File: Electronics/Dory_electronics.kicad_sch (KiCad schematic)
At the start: 12 parts, among them J1 Bateria 2s, J2 Conn_01x08, J3 Conn_01x08, J4 Motor B, J5 Motor A, J6 sensor IR, J7 VL53L0X_ESQUERDO, J9 VL53L0X_DIREITO, U1 LM7805_TO220

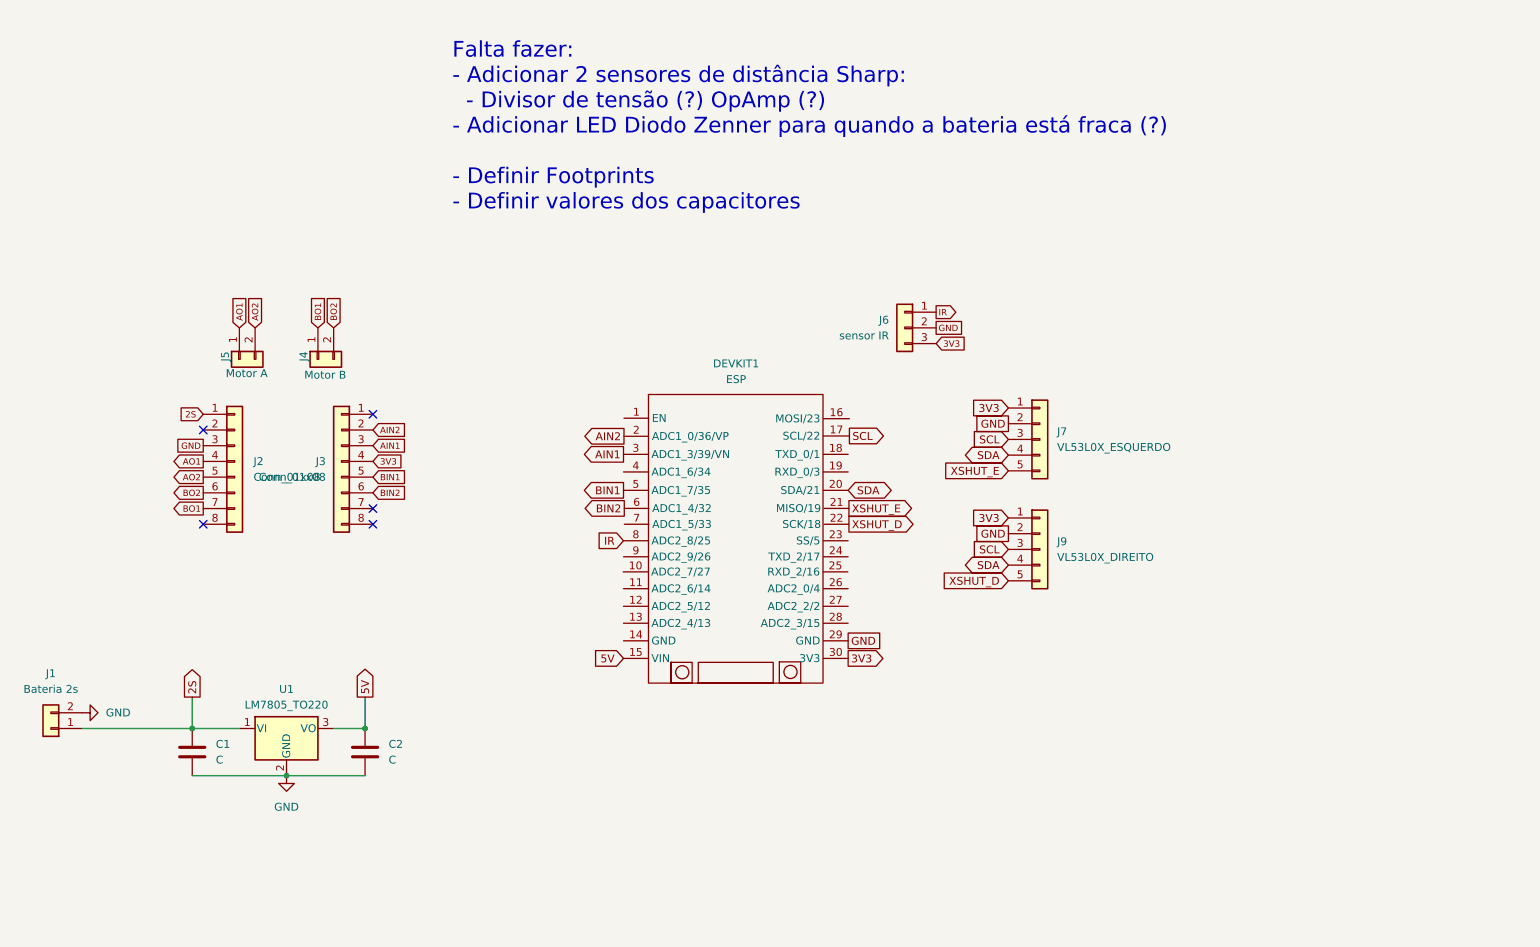
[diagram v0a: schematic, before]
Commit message: chore: revision of the PCB
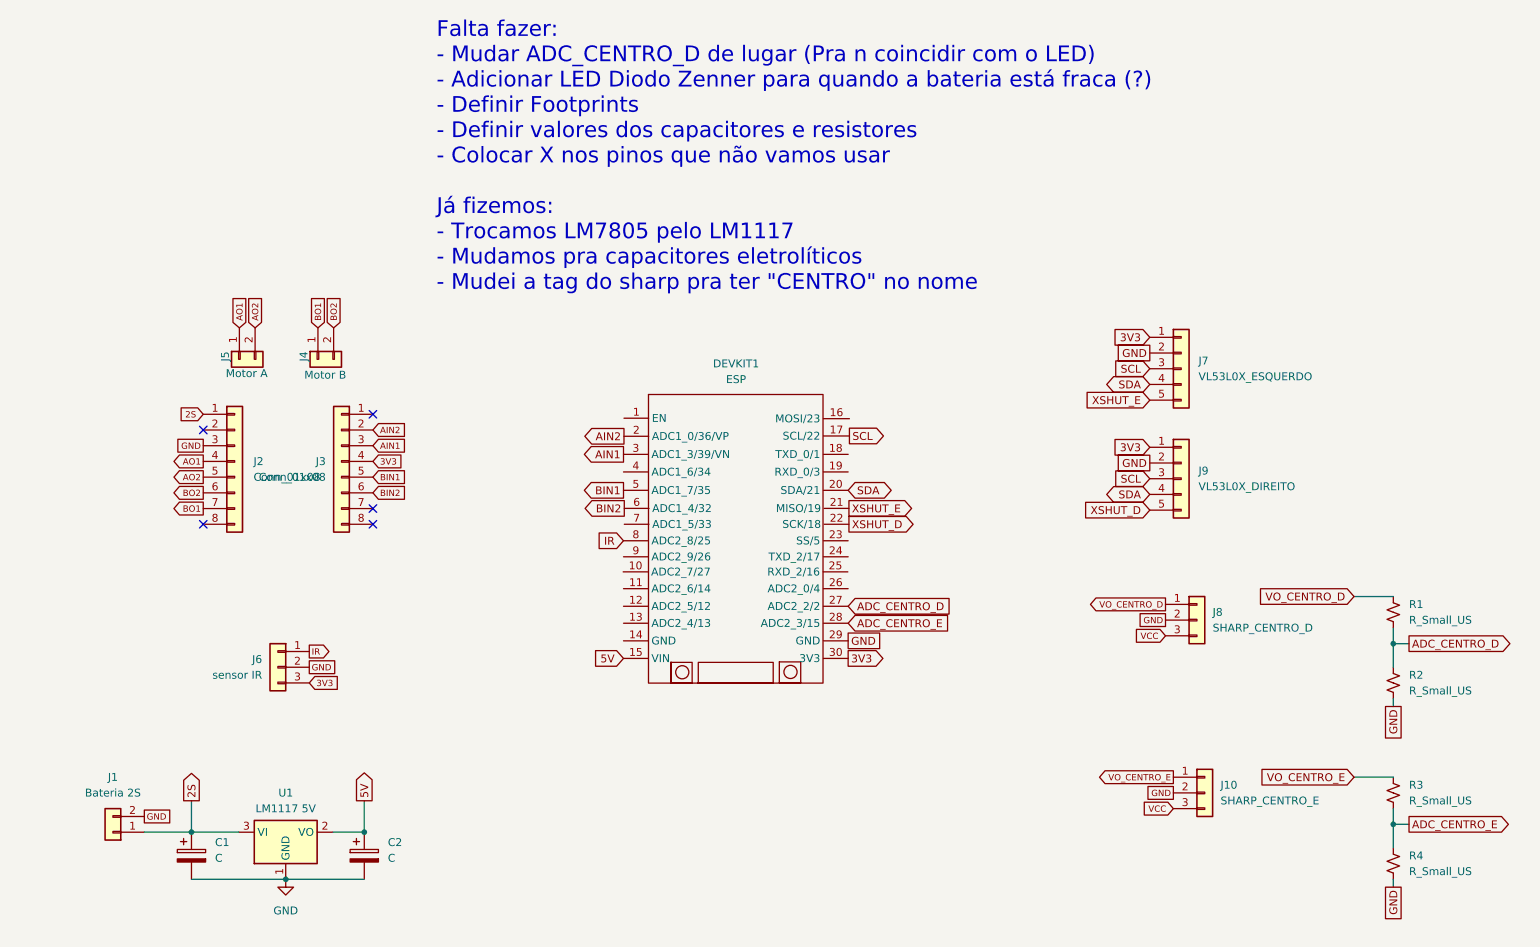
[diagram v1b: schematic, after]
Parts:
- added J10: SHARP_CENTRO_E, symbol Connector_Generic:Conn_01x03
- added J8: SHARP_CENTRO_D, symbol Connector_Generic:Conn_01x03
- added R1, R2, R3, R4: R_Small_US, symbol Device:R_Small_US
- C1, C2: symbol Device:C -> Device:C_Polarized
- J1: value Bateria 2s -> Bateria 2S
- U1: value LM7805_TO220 -> LM1117 5V; footprint Package_TO_SOT_THT:TO-220-3_Vertical -> Package_TO_SOT_THT:TO-220-3_Horizontal_TabDown; symbol Regulator_Linear:LM7805_TO220 -> Regulator_Linear:LM1117T-5.0
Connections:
- net 2S: now also U1.3 (VI); no longer U1.1 (VI)
- net 5V: now also U1.2 (VO); no longer U1.3 (VO)
- net GND: now also U1.1 (GND), J10.2 (Pin_2), J8.2 (Pin_2), R2.2, R4.2; no longer U1.2 (GND)
- net ADC_CENTRO_D: now reaches DEVKIT1.27 (ADC2_2/2)
- net ADC_CENTRO_D: now also R1.2, R2.1
- net ADC_CENTRO_E: now reaches DEVKIT1.28 (ADC2_3/15)
- net ADC_CENTRO_E: now also R3.2, R4.1
- new net VCC: J10.3 (Pin_3), J8.3 (Pin_3)
- new net VO_CENTRO_D: J8.1 (Pin_1), R1.1
- new net VO_CENTRO_E: J10.1 (Pin_1), R3.1
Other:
- note added: "Falta fazer: - Mudar ADC_CENTRO_D de lugar (Pra n coincidir com o LED) - Adicionar LED Diodo Zenner para quando a bateria está fraca (?) - Definir Footprints - Definir valores dos capacitores e resistores - Colocar X nos pinos que não vamos usar Já fizemos: - Trocamos LM7805 pelo LM1117 - Mudamos pra capacitores eletrolíticos - Mudei a tag do sharp pra ter "CENTRO" no nome"
- note removed: "Falta fazer: - Adicionar 2 sensores de distância Sharp: - Divisor de tensão (?) OpAmp (?) - Adicionar LED Diodo Zenner para quando a bateria está fraca (?) - Definir Footprints - Definir valores dos capacitores"
- moved on the sheet: J1, J6, J7, J9, U1
